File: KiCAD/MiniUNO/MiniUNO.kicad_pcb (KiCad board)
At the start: 2 copper layers, 22 x 18 mm, 21 parts, among them J1 USB_B_Micro, J2 Conn_01x11, J3 Conn_01x11, J4 Conn_01x07, U1 ATmega32U4-A, Y1 830108288709

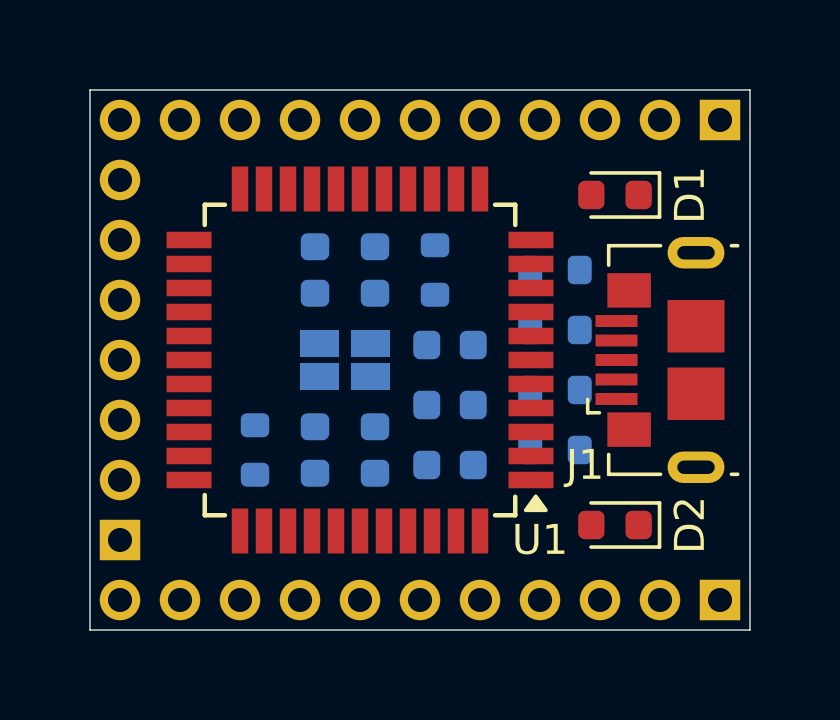
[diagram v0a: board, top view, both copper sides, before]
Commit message: Lots more work
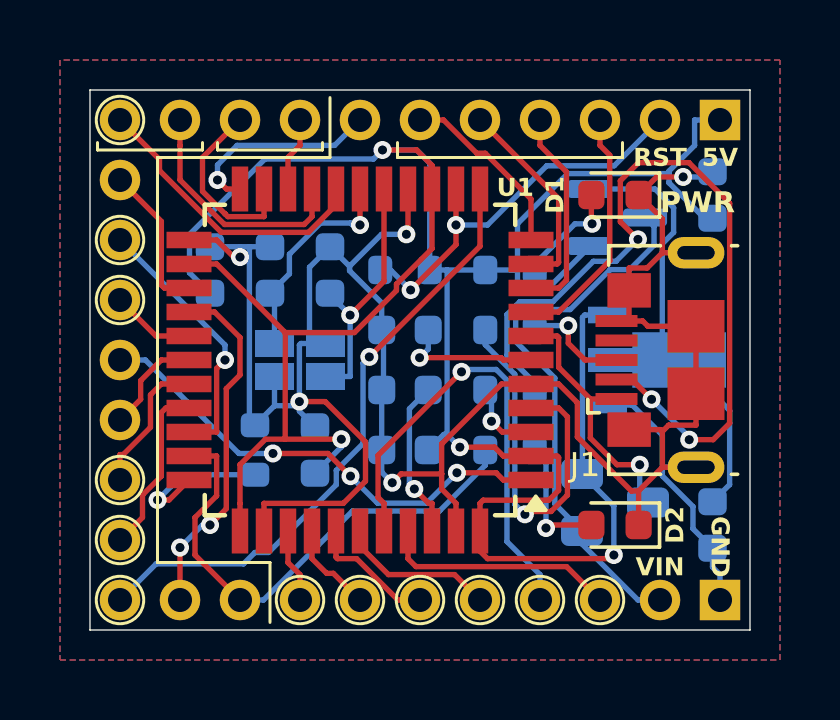
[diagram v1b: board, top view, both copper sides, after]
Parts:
- added C8: 1uF, Capacitor_SMD:C_0603_1608Metric, B.Cu at (11.8, -5.50)
- added C9: 1uF, Capacitor_SMD:C_0603_1608Metric, B.Cu at (11.8, 5.50)
- added IC1: AZ1117CR2-5.0TRG1, AZ1117CR2-5.0TRG1:AP738133Y13, B.Cu at (8.64, 0.00)
- added Q1: FDN340P, Package_TO_SOT_SMD:SuperSOT-3, B.Cu at (8.50, 4.75)
- added Q2: PMV48XP, Package_TO_SOT_SMD:SOT-23, B.Cu at (8.56, -4.75)
- moved J4 12.0 mm to (-8.00, -6.00), turned to 180 degrees
- moved C3 8.14 mm to (-5.00, -3.00)
- moved C5 1.58 mm to (1.50, 3.00)
- moved C6 1.58 mm to (1.50, -1.00)
- moved C7 1.58 mm to (1.50, 1.00)
- moved C1 1.50 mm to (-3.00, -3.00)
- moved C2 1.50 mm to (-1.00, -3.00)
- moved R1 1.50 mm to (5.00, -1.00)
- moved R2 1.50 mm to (5.00, 1.00)
- moved R5 1.50 mm to (5.00, -3.00)
- moved R6 1.50 mm to (5.00, 3.00)
- moved Y1 1.50 mm to (-2.00, 0.00)
- moved R4 1.00 mm to (1.50, -3.00), turned to 0 degrees
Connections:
- net Net-(U1-D+) renamed D+
- net Net-(U1-D-) renamed D-
- net Net-(U1-UCAP) renamed UCAP
- C3 pad 1: VCC -> +5V
- C4 pad 1: VCC -> +5V
- C5 pad 1: VCC -> +5V
- J1 pad 1: VCC -> VUSB
- J2 pad 1: VCC -> +5V
- J3 pad 2: AREF -> VIN
- R4 pad 2: VCC -> +5V
- R5 pad 1: VCC -> +5V
- U1 pad 14: VCC -> +5V
- U1 pad 2: VCC -> +5V
- U1 pad 24: VCC -> +5V
- U1 pad 34: VCC -> +5V
- U1 pad 44: VCC -> +5V
- U1 pad 7: VCC -> VUSB
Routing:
- net +5V: track 0.00 -> 89.8 mm, vias 0 -> 4
- net GND: track 0.00 -> 88.0 mm, vias 0 -> 5
- net Net-(J1-D-): track 0.00 -> 27.4 mm, vias 0 -> 3
- net D11: track 0.00 -> 20.6 mm, vias 0 -> 1
- net VIN: track 0.00 -> 18.5 mm
- net D13/USER_LED: track 0.00 -> 17.2 mm
- net Net-(IC1-IN): track 0.00 -> 16.3 mm
- net D7: track 0.00 -> 16.2 mm, vias 0 -> 3
- net A4: track 0.00 -> 16.0 mm, vias 0 -> 1
- net RESET: track 0.00 -> 13.5 mm, vias 0 -> 2
- net D+: track 0.00 -> 12.3 mm, vias 0 -> 1
- net D12: track 0.00 -> 11.8 mm, vias 0 -> 2
- net D3/SCL: track 0.00 -> 9.88 mm
- net VUSB: track 0.00 -> 8.99 mm, vias 0 -> 1
- net D5: track 0.00 -> 8.89 mm, vias 0 -> 1
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- added copper zone on B.Cu, net GND
- added copper zone on F.Cu, net GND
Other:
- board text added: "5V"
- board text added: "GND"
- board text added: "PWR"
- board text added: "RST"
- board text added: "VIN"
